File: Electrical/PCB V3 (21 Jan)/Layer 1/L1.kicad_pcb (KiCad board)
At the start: 2 copper layers, 178 x 170 mm, 198 parts, among them J1 Conn_01x02, J3 Conn_01x02, SW1 SW_SPDT, U2 CD74HC4067SM, U3 CD74HC4067SM, U4 XT30UPB-M, U5 113991054

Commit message: finished l1?
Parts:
- J1, J3, TP1: footprint Connector_PinHeader_1.00mm:PinHeader_1x02_P1.00mm_Vertical -> Connector_PinHeader_2.54mm:PinHeader_1x02_P2.54mm_Vertical
- R33, R34: footprint Resistor_SMD:R_0201_0603Metric -> Resistor_SMD:R_0603_1608Metric
- moved U4 245.9 mm to (83.2, 35.6), turned to -45 degrees
- moved U5 196.2 mm to (113.8, 37.8)
- moved SW1 180.9 mm to (89.1, 32.3), turned to 45 degrees
- moved TP1 174.7 mm to (97.7, 37.0), turned to 180 degrees
- moved J3 167.2 mm to (102.2, 36.8), turned to 180 degrees
- moved R33 163.9 mm to (109.0, 29.4), turned to -90 degrees
- moved R34 162.8 mm to (109.1, 33.7), turned to 90 degrees
- moved J1 162.2 mm to (102.2, 43.1), turned to 180 degrees
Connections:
- L10 pad 1: Net-(LED1-A) -> Net-(LED10-A)
- L10 pad 2: Net-(L1-Pad2) -> Net-(L10-Pad2)
- L11 pad 1: Net-(LED1-A) -> Net-(LED11-A)
- L11 pad 2: Net-(L1-Pad2) -> Net-(L11-Pad2)
- L12 pad 1: Net-(LED1-A) -> Net-(LED12-A)
- L12 pad 2: Net-(L1-Pad2) -> Net-(L12-Pad2)
- L13 pad 1: Net-(LED1-A) -> Net-(LED13-A)
- L13 pad 2: Net-(L1-Pad2) -> Net-(L13-Pad2)
- L14 pad 1: Net-(LED1-A) -> Net-(LED14-A)
- L14 pad 2: Net-(L1-Pad2) -> Net-(L14-Pad2)
- L15 pad 1: Net-(LED1-A) -> Net-(LED15-A)
- L15 pad 2: Net-(L1-Pad2) -> Net-(L15-Pad2)
- L16 pad 1: Net-(LED1-A) -> Net-(LED16-A)
- L16 pad 2: Net-(L1-Pad2) -> Net-(L16-Pad2)
- L17 pad 1: Net-(LED1-A) -> Net-(LED17-A)
- L17 pad 2: Net-(L1-Pad2) -> Net-(L17-Pad2)
- L18 pad 1: Net-(LED1-A) -> Net-(LED18-A)
- L18 pad 2: Net-(L1-Pad2) -> Net-(L18-Pad2)
- L19 pad 1: Net-(LED1-A) -> Net-(LED19-A)
- L19 pad 2: Net-(L1-Pad2) -> Net-(L19-Pad2)
- L2 pad 1: Net-(LED1-A) -> Net-(LED2-A)
- L2 pad 2: Net-(L1-Pad2) -> Net-(L2-Pad2)
- L20 pad 1: Net-(LED1-A) -> Net-(LED20-A)
- L20 pad 2: Net-(L1-Pad2) -> Net-(L20-Pad2)
- L21 pad 1: Net-(LED1-A) -> Net-(LED21-A)
- L21 pad 2: Net-(L1-Pad2) -> Net-(L21-Pad2)
- L22 pad 1: Net-(LED1-A) -> Net-(LED22-A)
- L22 pad 2: Net-(L1-Pad2) -> Net-(L22-Pad2)
- L23 pad 1: Net-(LED1-A) -> Net-(LED23-A)
- L23 pad 2: Net-(L1-Pad2) -> Net-(L23-Pad2)
- L24 pad 1: Net-(LED1-A) -> Net-(LED24-A)
- L24 pad 2: Net-(L1-Pad2) -> Net-(L24-Pad2)
- L25 pad 1: Net-(LED1-A) -> Net-(LED25-A)
- L25 pad 2: Net-(L1-Pad2) -> Net-(L25-Pad2)
- L26 pad 1: Net-(LED1-A) -> Net-(LED26-A)
- L26 pad 2: Net-(L1-Pad2) -> Net-(L26-Pad2)
- L27 pad 1: Net-(LED1-A) -> Net-(LED27-A)
- L27 pad 2: Net-(L1-Pad2) -> Net-(L27-Pad2)
- L28 pad 1: Net-(LED1-A) -> Net-(LED28-A)
- L28 pad 2: Net-(L1-Pad2) -> Net-(L28-Pad2)
- L29 pad 1: Net-(LED1-A) -> Net-(LED29-A)
- L29 pad 2: Net-(L1-Pad2) -> Net-(L29-Pad2)
- L3 pad 1: Net-(LED1-A) -> Net-(LED3-A)
- L3 pad 2: Net-(L1-Pad2) -> Net-(L3-Pad2)
- L30 pad 1: Net-(LED1-A) -> Net-(LED30-A)
- L30 pad 2: Net-(L1-Pad2) -> Net-(L30-Pad2)
- L31 pad 1: Net-(LED1-A) -> Net-(LED31-A)
- L31 pad 2: Net-(L1-Pad2) -> Net-(L31-Pad2)
- L32 pad 1: Net-(LED1-A) -> Net-(LED32-A)
- L32 pad 2: Net-(L1-Pad2) -> Net-(L32-Pad2)
- L4 pad 1: Net-(LED1-A) -> Net-(LED4-A)
- L4 pad 2: Net-(L1-Pad2) -> Net-(L4-Pad2)
- L5 pad 1: Net-(LED1-A) -> Net-(LED5-A)
- L5 pad 2: Net-(L1-Pad2) -> Net-(L5-Pad2)
- L6 pad 1: Net-(LED1-A) -> Net-(LED6-A)
- L6 pad 2: Net-(L1-Pad2) -> Net-(L6-Pad2)
- L7 pad 1: Net-(LED1-A) -> Net-(LED7-A)
- L7 pad 2: Net-(L1-Pad2) -> Net-(L7-Pad2)
- L8 pad 1: Net-(LED1-A) -> Net-(LED8-A)
- L8 pad 2: Net-(L1-Pad2) -> Net-(L8-Pad2)
- L9 pad 1: Net-(LED1-A) -> Net-(LED9-A)
- L9 pad 2: Net-(L1-Pad2) -> Net-(L9-Pad2)
- LED10 pad 2: Net-(LED1-A) -> Net-(LED10-A)
- LED11 pad 2: Net-(LED1-A) -> Net-(LED11-A)
- LED12 pad 2: Net-(LED1-A) -> Net-(LED12-A)
- LED13 pad 2: Net-(LED1-A) -> Net-(LED13-A)
- LED14 pad 2: Net-(LED1-A) -> Net-(LED14-A)
- LED15 pad 2: Net-(LED1-A) -> Net-(LED15-A)
- LED16 pad 2: Net-(LED1-A) -> Net-(LED16-A)
- LED17 pad 2: Net-(LED1-A) -> Net-(LED17-A)
- LED18 pad 2: Net-(LED1-A) -> Net-(LED18-A)
- LED19 pad 2: Net-(LED1-A) -> Net-(LED19-A)
- LED2 pad 2: Net-(LED1-A) -> Net-(LED2-A)
- LED20 pad 2: Net-(LED1-A) -> Net-(LED20-A)
- LED21 pad 2: Net-(LED1-A) -> Net-(LED21-A)
- LED22 pad 2: Net-(LED1-A) -> Net-(LED22-A)
- LED23 pad 2: Net-(LED1-A) -> Net-(LED23-A)
- LED24 pad 2: Net-(LED1-A) -> Net-(LED24-A)
- LED25 pad 2: Net-(LED1-A) -> Net-(LED25-A)
- LED26 pad 2: Net-(LED1-A) -> Net-(LED26-A)
- LED27 pad 2: Net-(LED1-A) -> Net-(LED27-A)
- LED28 pad 2: Net-(LED1-A) -> Net-(LED28-A)
- LED29 pad 2: Net-(LED1-A) -> Net-(LED29-A)
- LED3 pad 2: Net-(LED1-A) -> Net-(LED3-A)
- LED30 pad 2: Net-(LED1-A) -> Net-(LED30-A)
- LED31 pad 2: Net-(LED1-A) -> Net-(LED31-A)
- LED32 pad 2: Net-(LED1-A) -> Net-(LED32-A)
- LED4 pad 2: Net-(LED1-A) -> Net-(LED4-A)
- LED5 pad 2: Net-(LED1-A) -> Net-(LED5-A)
- LED6 pad 2: Net-(LED1-A) -> Net-(LED6-A)
- LED7 pad 2: Net-(LED1-A) -> Net-(LED7-A)
- LED8 pad 2: Net-(LED1-A) -> Net-(LED8-A)
- LED9 pad 2: Net-(LED1-A) -> Net-(LED9-A)
- R10 pad 2: Net-(L1-Pad2) -> Net-(L10-Pad2)
- R11 pad 2: Net-(L1-Pad2) -> Net-(L11-Pad2)
- R12 pad 2: Net-(L1-Pad2) -> Net-(L12-Pad2)
- R13 pad 2: Net-(L1-Pad2) -> Net-(L13-Pad2)
- R14 pad 2: Net-(L1-Pad2) -> Net-(L14-Pad2)
- R15 pad 2: Net-(L1-Pad2) -> Net-(L15-Pad2)
- R16 pad 2: Net-(L1-Pad2) -> Net-(L16-Pad2)
- R17 pad 2: Net-(L1-Pad2) -> Net-(L17-Pad2)
- R18 pad 2: Net-(L1-Pad2) -> Net-(L18-Pad2)
- R19 pad 2: Net-(L1-Pad2) -> Net-(L19-Pad2)
- R2 pad 2: Net-(L1-Pad2) -> Net-(L2-Pad2)
- R20 pad 2: Net-(L1-Pad2) -> Net-(L20-Pad2)
- R21 pad 2: Net-(L1-Pad2) -> Net-(L21-Pad2)
- R22 pad 2: Net-(L1-Pad2) -> Net-(L22-Pad2)
- R23 pad 2: Net-(L1-Pad2) -> Net-(L23-Pad2)
- R24 pad 2: Net-(L1-Pad2) -> Net-(L24-Pad2)
- R25 pad 2: Net-(L1-Pad2) -> Net-(L25-Pad2)
- R26 pad 2: Net-(L1-Pad2) -> Net-(L26-Pad2)
- R27 pad 2: Net-(L1-Pad2) -> Net-(L27-Pad2)
- R28 pad 2: Net-(L1-Pad2) -> Net-(L28-Pad2)
- R29 pad 2: Net-(L1-Pad2) -> Net-(L29-Pad2)
- R3 pad 2: Net-(L1-Pad2) -> Net-(L3-Pad2)
- R30 pad 2: Net-(L1-Pad2) -> Net-(L30-Pad2)
- R31 pad 2: Net-(L1-Pad2) -> Net-(L31-Pad2)
- R32 pad 2: Net-(L1-Pad2) -> Net-(L32-Pad2)
- R33 pad 2: /Mux Com (1-16) -> /Mux Com (17-32)
- R34 pad 2: /Mux Com (17-32) -> /Mux Com (1-16)
- R4 pad 2: Net-(L1-Pad2) -> Net-(L4-Pad2)
- R5 pad 2: Net-(L1-Pad2) -> Net-(L5-Pad2)
- R6 pad 2: Net-(L1-Pad2) -> Net-(L6-Pad2)
- R7 pad 2: Net-(L1-Pad2) -> Net-(L7-Pad2)
- R8 pad 2: Net-(L1-Pad2) -> Net-(L8-Pad2)
- R9 pad 2: Net-(L1-Pad2) -> Net-(L9-Pad2)
- U2 pad 1: /Mux Com (1-16) -> /Mux Com (17-32)
- U3 pad 1: /Mux Com (17-32) -> /Mux Com (1-16)
- U5 pad 1: /Mux Com (1-16) -> /Mux Com (17-32)
- U5 pad 2: /Mux Com (17-32) -> /Mux Com (1-16)
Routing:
- net +3V3: track 0.00 -> 142.5 mm
- net /Mux Com (17-32): track 0.00 -> 95.9 mm, vias 0 -> 1
- net /Mux Com (1-16): track 0.00 -> 92.1 mm, vias 0 -> 1
- net /S0: track 0.00 -> 89.8 mm, vias 0 -> 3
- net /S2: track 0.00 -> 84.4 mm, vias 0 -> 3
- net /S1: track 0.00 -> 84.2 mm, vias 0 -> 3
- net /S3: track 0.00 -> 79.3 mm, vias 0 -> 3
- net Net-(LED1-A): track 72.5 -> 2.27 mm
- net Net-(L1-Pad2): track 61.2 -> 1.91 mm
- net Net-(U2-I5): track 0.00 -> 57.1 mm
- net Net-(U2-I4): track 0.00 -> 55.5 mm
- net Net-(U2-I3): track 0.00 -> 54.8 mm
- net Net-(U2-I0): track 0.00 -> 50.8 mm
- net Net-(U2-I12): track 0.00 -> 50.6 mm
- net Net-(U2-I6): track 0.00 -> 50.3 mm
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
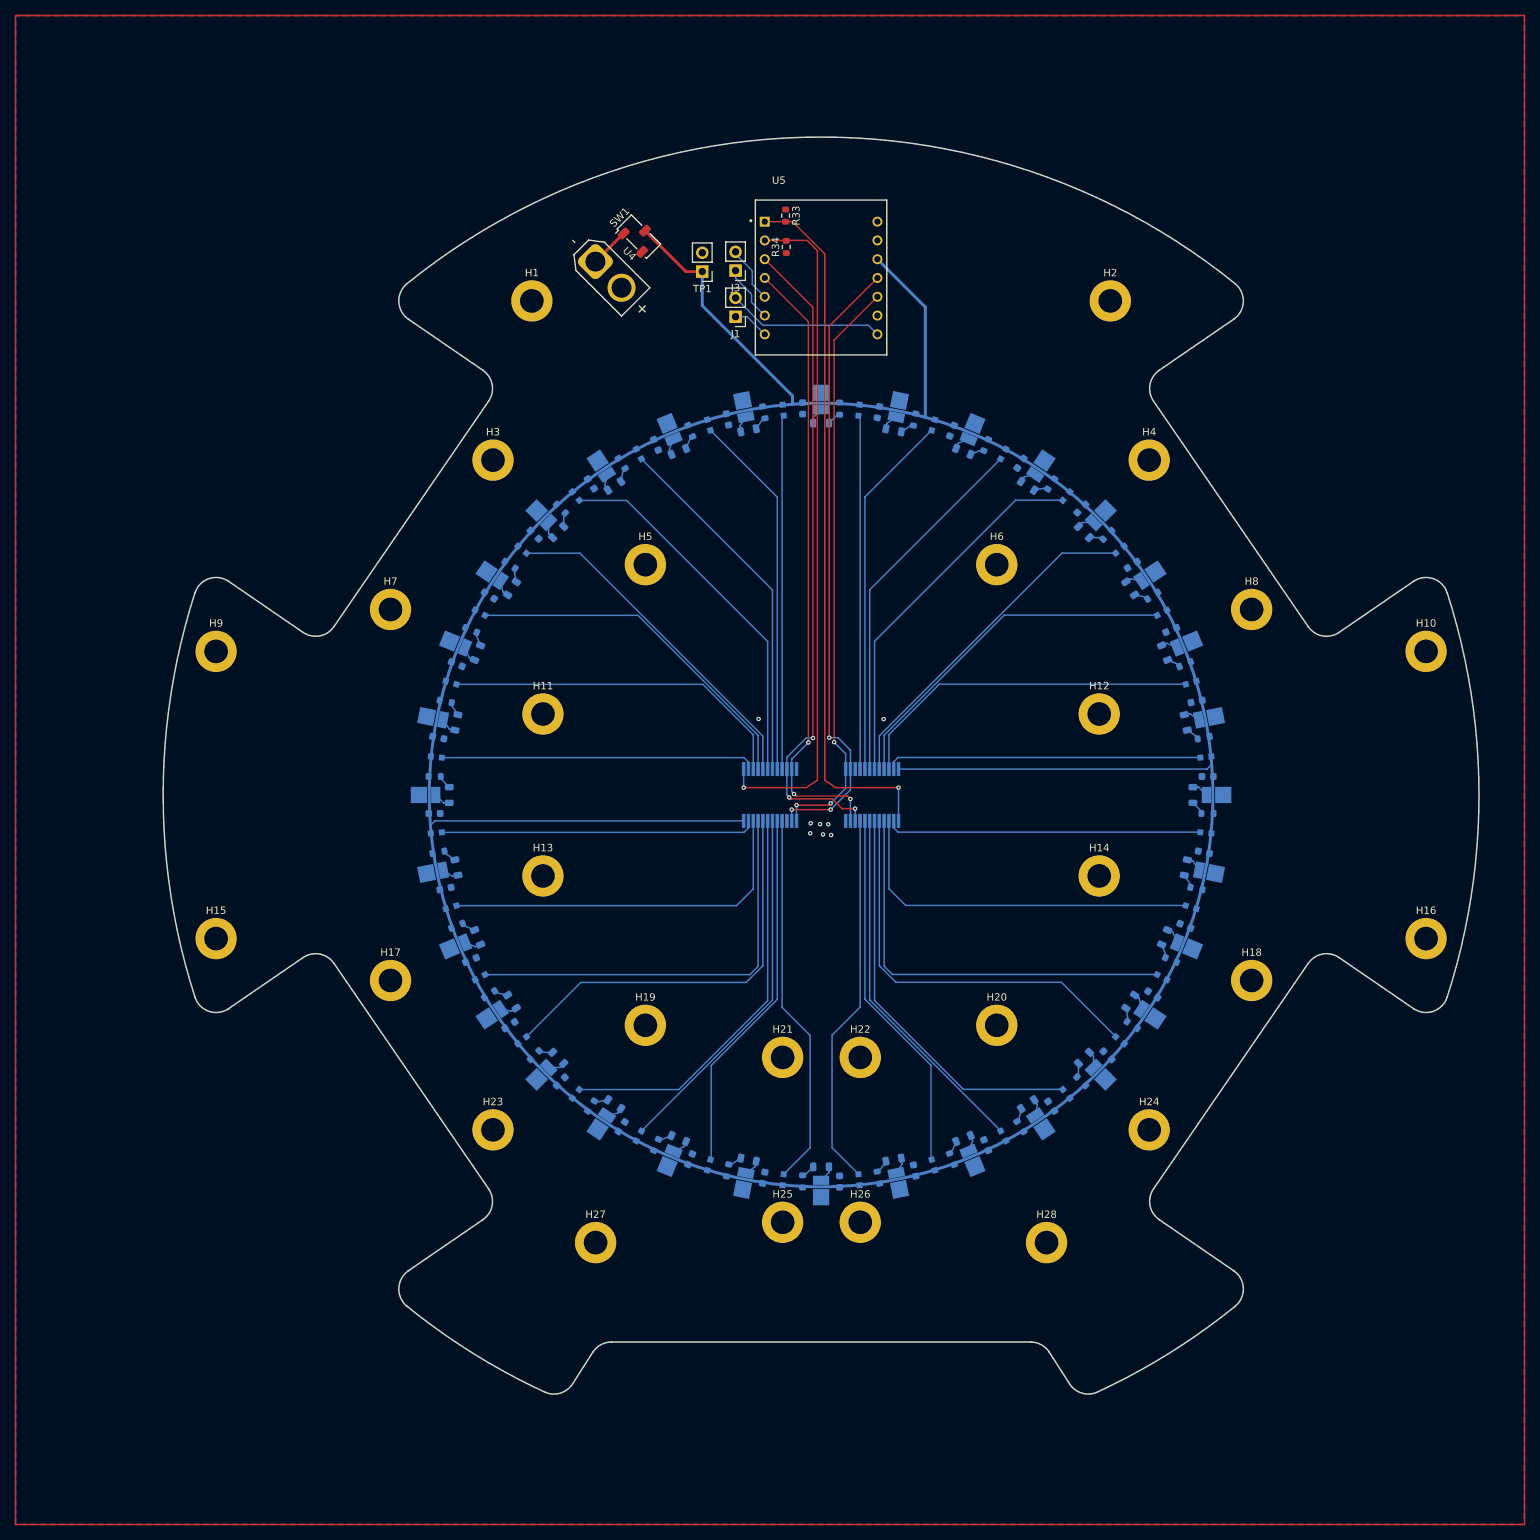
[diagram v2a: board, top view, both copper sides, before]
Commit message: finished layer1?
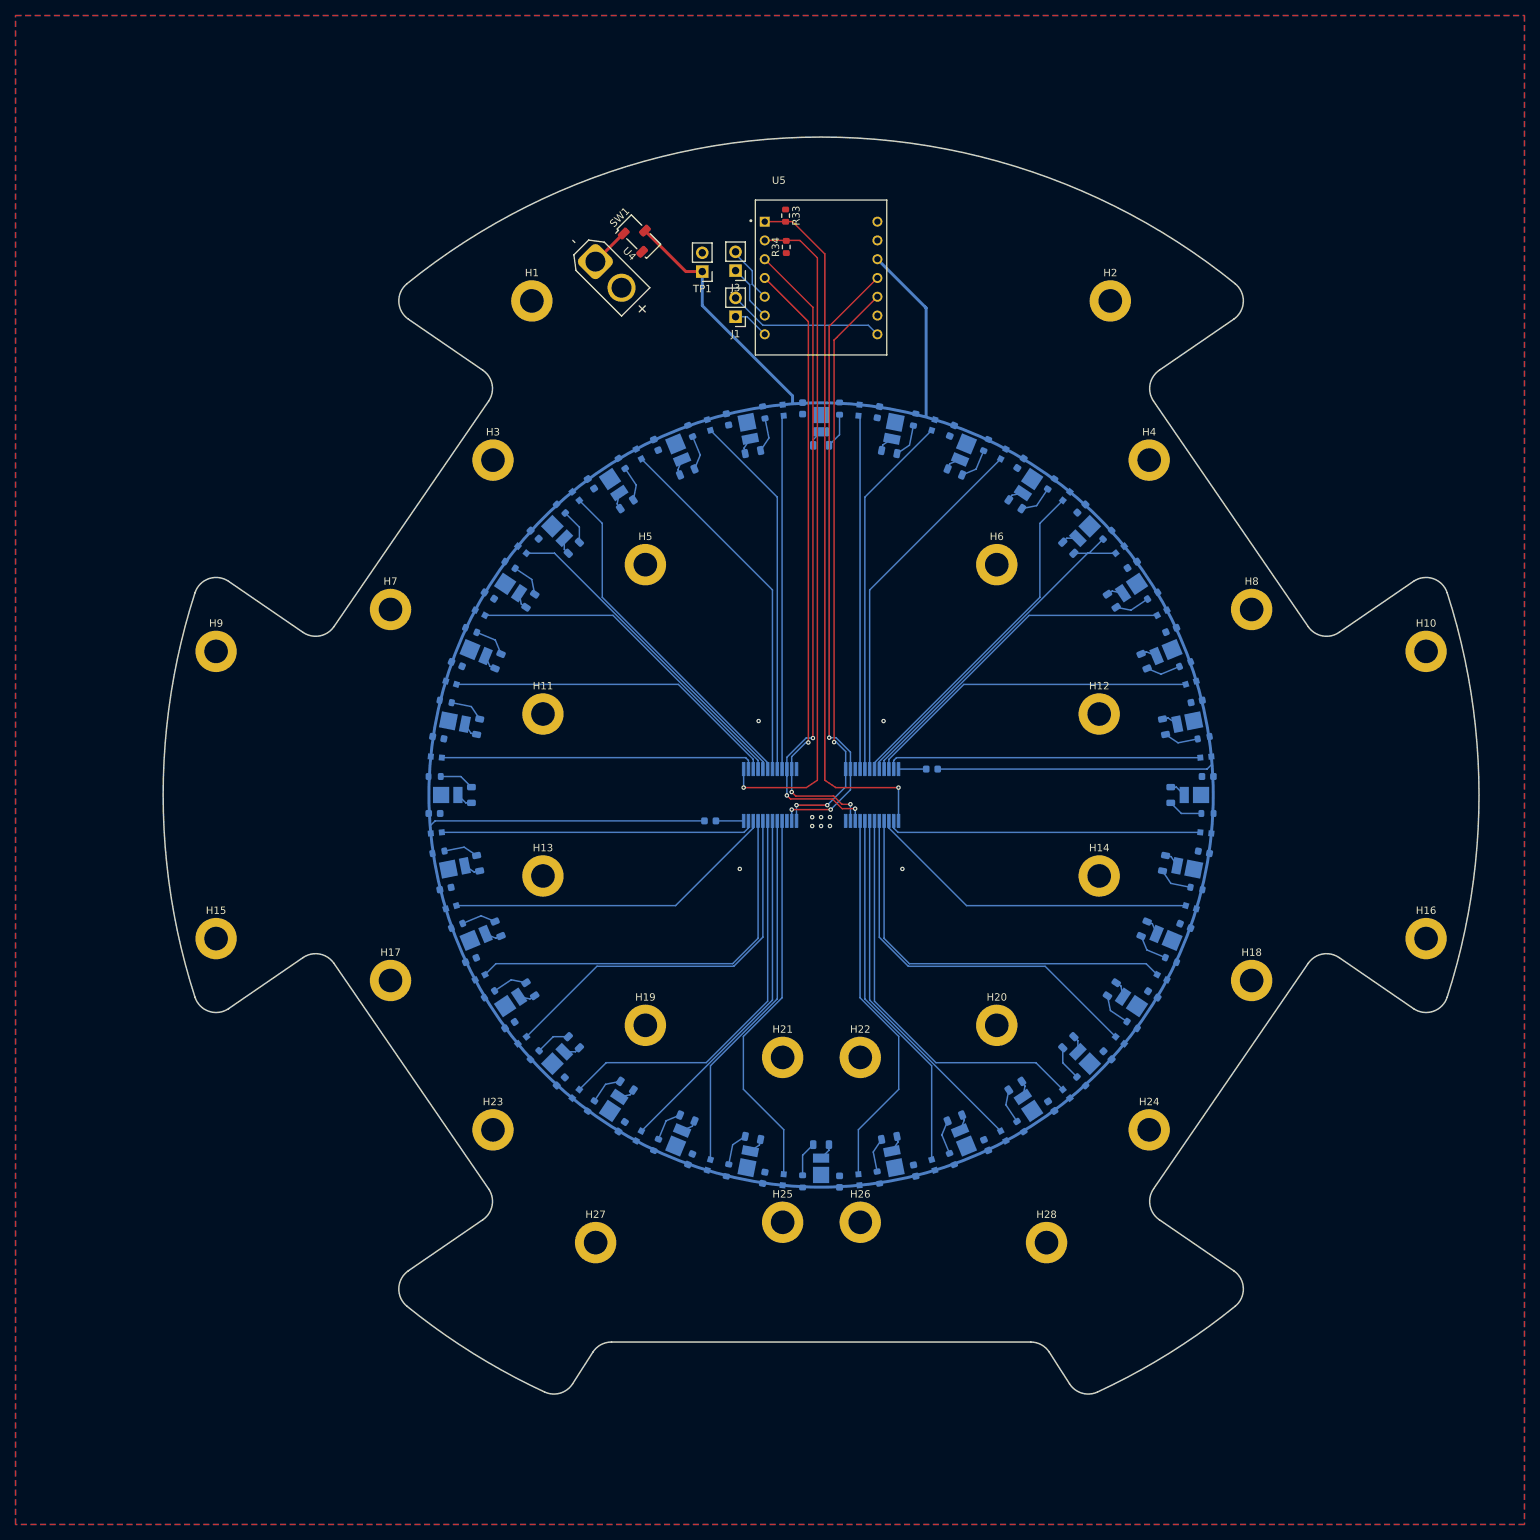
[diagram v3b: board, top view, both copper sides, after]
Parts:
- added C33: C, Capacitor_SMD:C_0603_1608Metric, B.Cu at (98.8, 111.3)
- added C34: C, Capacitor_SMD:C_0603_1608Metric, B.Cu at (128.8, 104.3)
- moved L24 3.00 mm to (160.2, 117.0)
- moved LED16 3.00 mm to (103.9, 157.3)
- moved LED32 3.00 mm to (123.6, 58.3)
- moved LED8 3.00 mm to (64.2, 97.9)
- moved L32 3.00 mm to (123.0, 61.4)
- moved L8 3.00 mm to (67.4, 98.6)
- moved L16 3.00 mm to (104.5, 154.2)
- moved LED24 3.00 mm to (163.3, 117.6)
- moved L23 3.00 mm to (157.5, 125.9)
- moved L27 3.00 mm to (157.5, 89.7)
- moved LED11 3.00 mm to (67.1, 127.1)
- moved LED7 3.00 mm to (67.1, 88.5)
- moved L3 3.00 mm to (95.7, 64.1)
- moved LED3 3.00 mm to (94.4, 61.1)
- moved LED31 3.00 mm to (133.1, 61.1)
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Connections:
- U2 pad 24: +3V3 -> Net-(U2-VCC)
- U3 pad 24: +3V3 -> Net-(U3-VCC)
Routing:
- net Net-(U2-I11): track 46.7 -> 0.00 mm
- net Net-(U3-I4): track 46.7 -> 89.3 mm
- net +3V3: track 142.5 -> 131.5 mm
- net Net-(U3-I9): track 50.3 -> 45.5 mm
- net Net-(U2-I6): track 50.3 -> 45.5 mm
- net Net-(U2-VCC): track 0.00 -> 3.76 mm
- net Net-(U3-VCC): track 0.00 -> 3.75 mm
- net Net-(U3-I3): track 50.6 -> 46.9 mm
- net Net-(U2-I12): track 50.6 -> 46.9 mm
- net Net-(L15-Pad2): track 1.91 -> 5.03 mm
- net Net-(L7-Pad2): track 1.91 -> 5.03 mm
- net Net-(L23-Pad2): track 1.91 -> 5.03 mm
- net Net-(L31-Pad2): track 1.91 -> 5.03 mm
- net Net-(L16-Pad2): track 1.91 -> 5.03 mm
- net Net-(L24-Pad2): track 1.91 -> 5.03 mm
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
